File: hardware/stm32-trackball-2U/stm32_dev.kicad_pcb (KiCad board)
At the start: 2 copper layers, 38.5 x 19 mm, 48 parts, among them J1 USB_C_Receptacle_USB2.0, J2 USB, Q3 DTC123J, SW1 SW_Push, SW2 BIG, SW3 SW_Push, SW4 BIG, T1 Trackball, U1 AP2112K-3.3, U2 USBLC6-2SC6, U3 STM32F042G6Ux, U4 AN48840B, U5 AN48840B, U6 AN48840B, U7 AN48840B

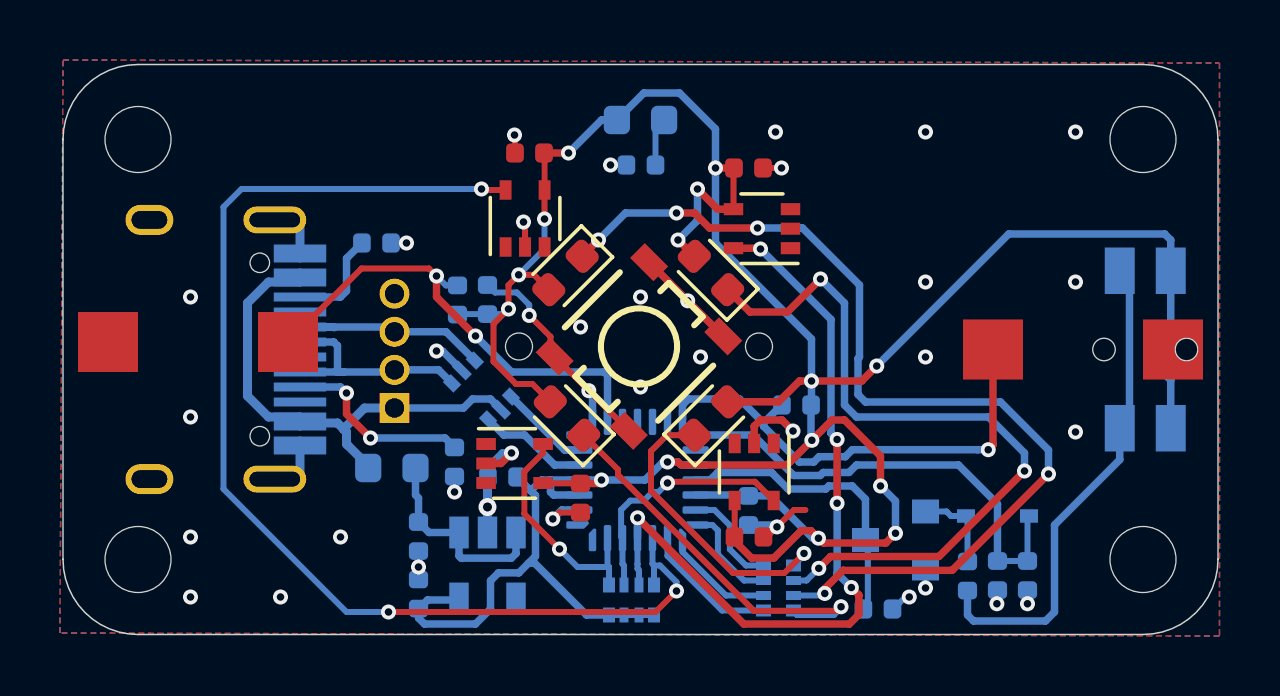
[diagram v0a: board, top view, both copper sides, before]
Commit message: Fast forward to KiCad 7 ;)
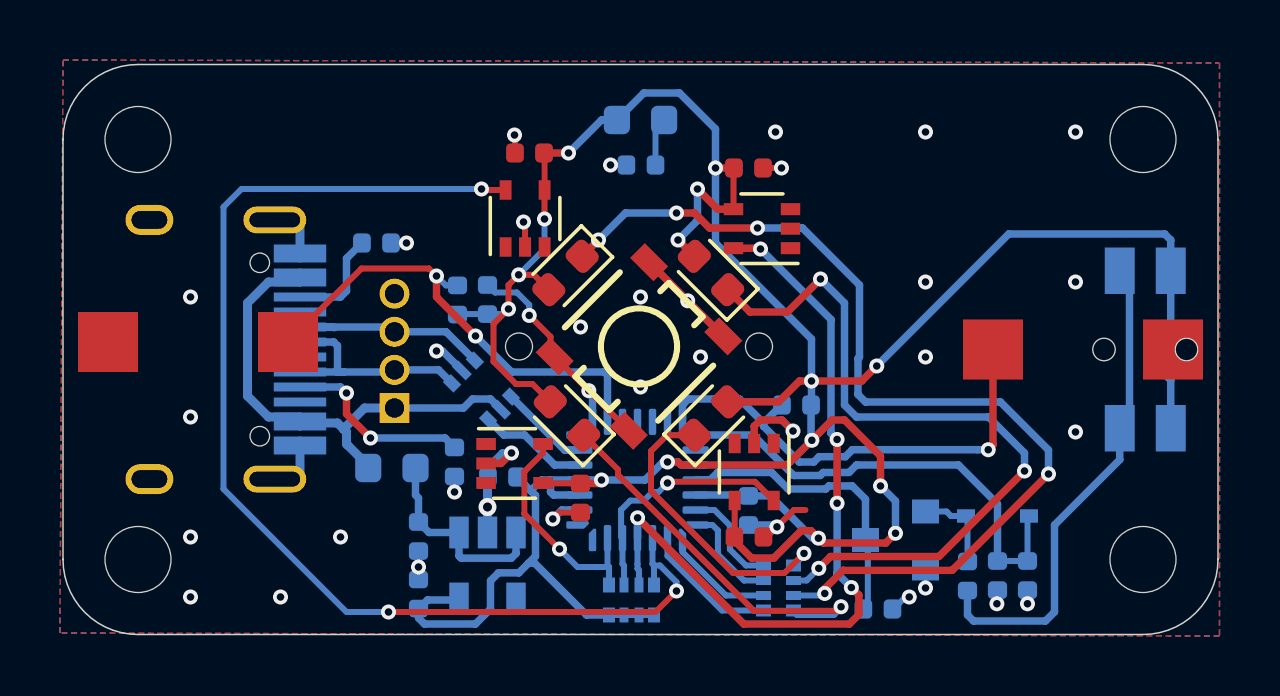
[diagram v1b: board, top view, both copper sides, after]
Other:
- net class Default removed
